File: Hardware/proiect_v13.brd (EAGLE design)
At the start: 160 x 93.7 mm, 103 parts, among them IC1 XC6220A331MR-G, IC2 BD5229G-TR, J1 SAMACSYS_PARTS_USB4110-GF-A, J2 112A-TAAR-R03_ATTEND, J3 FH34SRJ-24S-0.5SH_99_, J4 QWIIC_RIGHT_ANGLE, Q1 20V/4.2A/52mΩ/1.4W, Q2 SI1308EDL-T1-GE3, Q3 20V/4.2A/52mΩ/1.4W, U1 ESP32_WROVER_SPARKFUN-IC-POWE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, U2 ESP32-C6-WROOM-1-N8, U3 ESP32_WROVER_BME680_BME680, U4 MAX17048G+T10, U5 DS3231SN#, U6 W25Q512JVEIQ

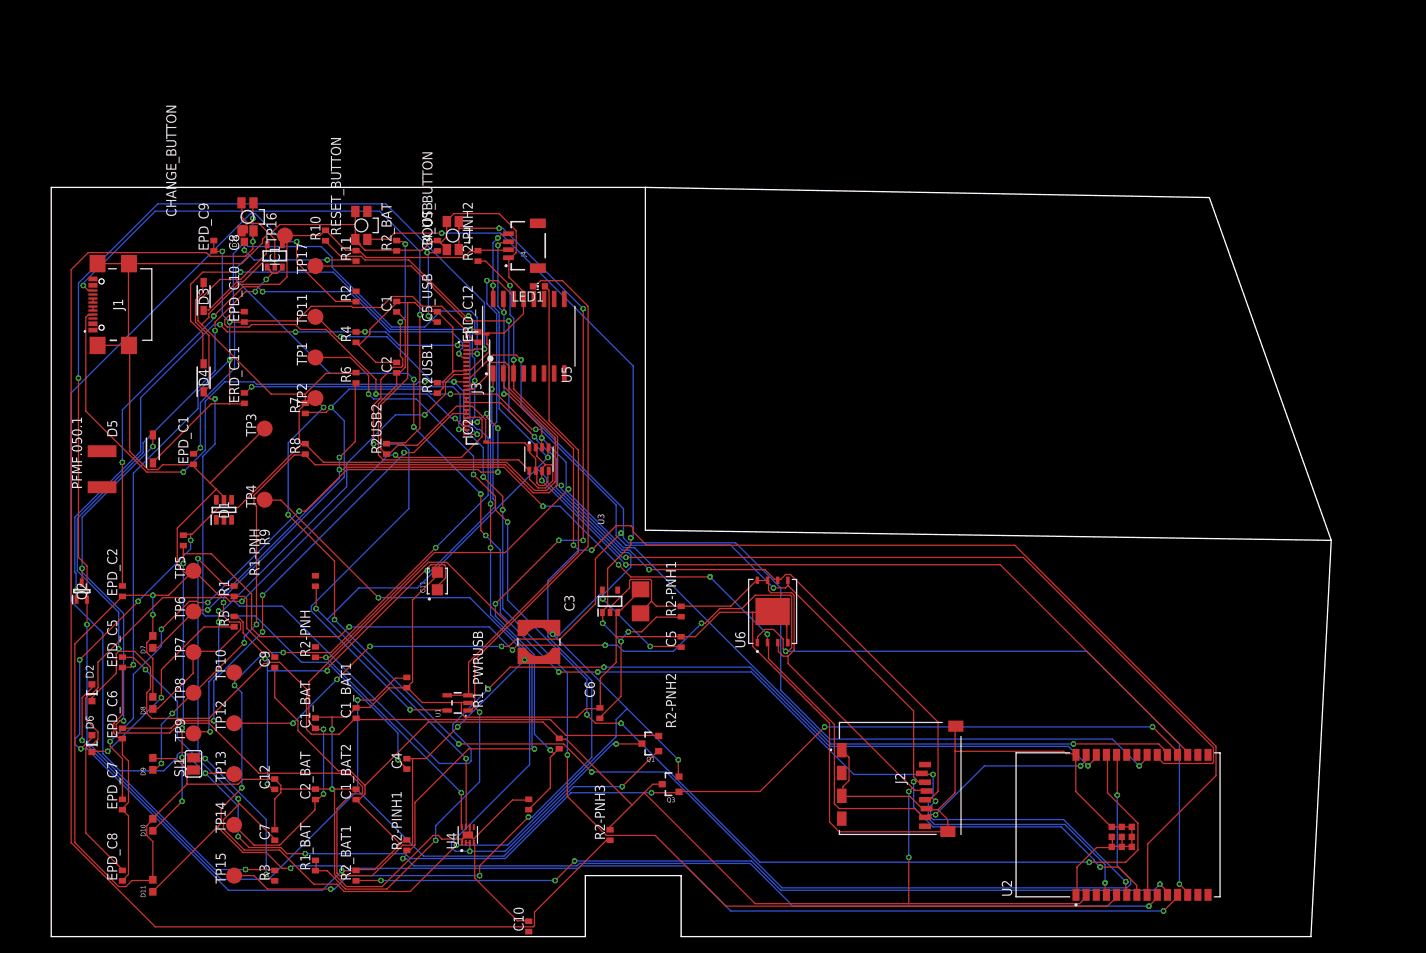
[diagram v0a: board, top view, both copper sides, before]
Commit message: Add files via upload
improved pcb
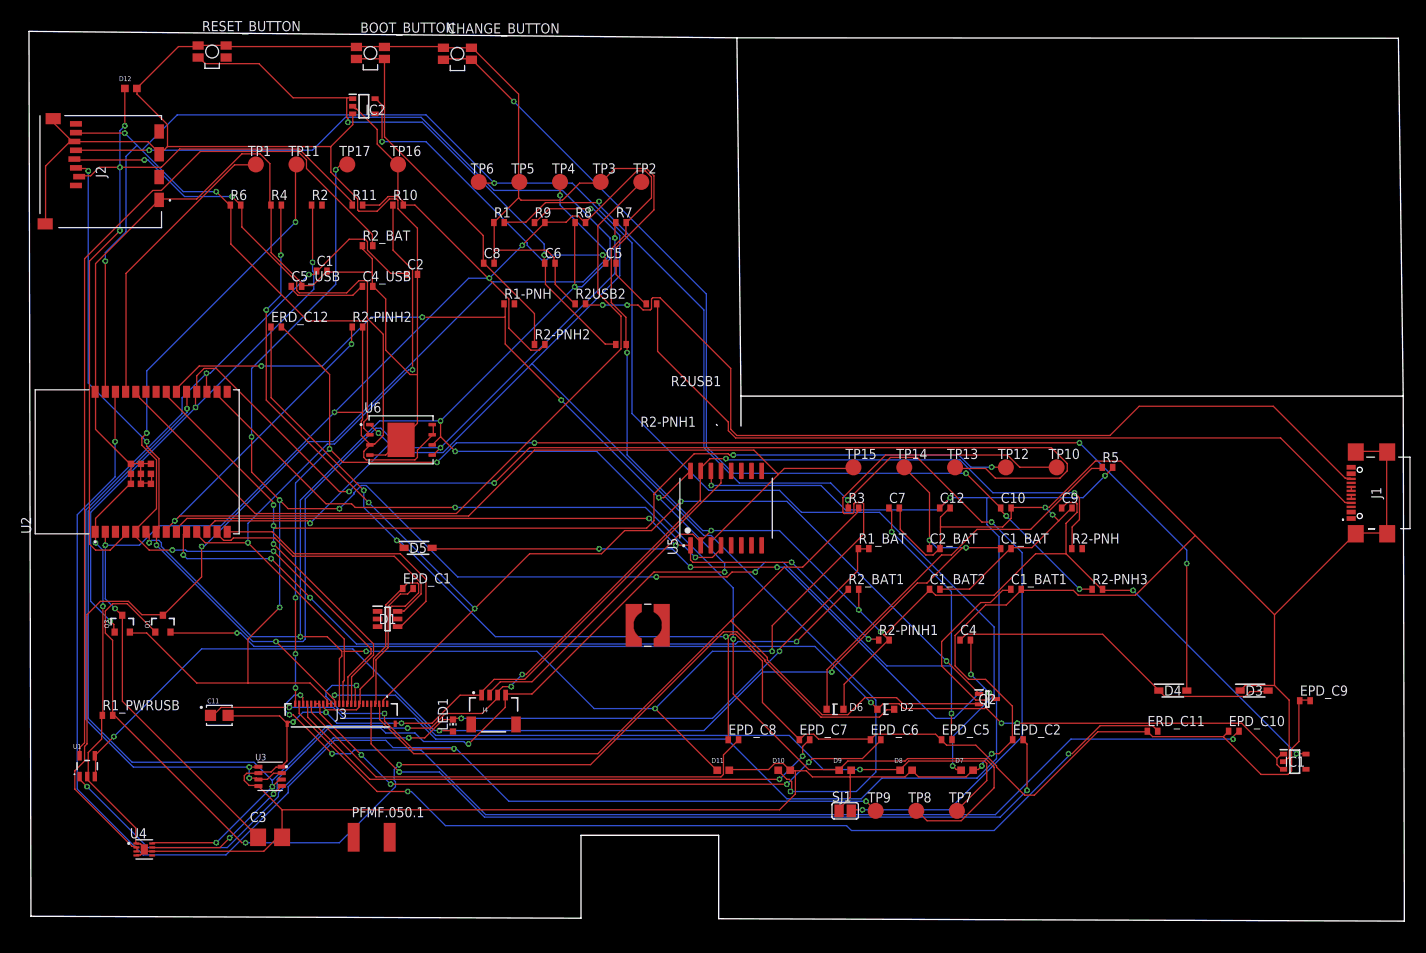
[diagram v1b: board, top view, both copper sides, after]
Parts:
- moved J1 159.0 mm to (168.7, 51.7)
- moved EPD_C9 147.8 mm to (159.2, 25.7), turned to 0 degrees
- moved IC1 142.3 mm to (158.0, 18.1), turned to 0 degrees
- moved D3 140.2 mm to (152.9, 26.9), turned to 0 degrees
- moved J2 139.1 mm to (5.63, 98.9), turned to 270 degrees
- moved EPD_C10 134.1 mm to (150.4, 21.9), turned to 0 degrees
- moved U2 130.7 mm to (13.3, 55.5)
- moved D4 127.3 mm to (142.7, 26.9), turned to 0 degrees
- moved ERD_C11 120.9 mm to (140.2, 21.9), turned to 0 degrees
- moved Q2 114.0 mm to (119.6, 25.9), turned to 0 degrees
- moved EPD_C2 113.5 mm to (123.4, 20.8), turned to 0 degrees
- moved R5 110.9 mm to (134.6, 54.8), turned to 0 degrees
- moved TP10 106.0 mm to (128.2, 54.8), turned to 0 degrees
- moved EPD_C5 103.5 mm to (114.5, 20.8), turned to 0 degrees
- moved D7 103.0 mm to (117.0, 17.0), turned to 0 degrees
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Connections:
- removed net RTC_RTS: U2.16
- removed net USR_D+: U2.14
- removed net USR_D-: U2.13
- net RTC_RST: now also U2.16
- net USB_D+: now also U2.14
- net USB_D-: now also U2.13
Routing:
- net GND: track 689.3 -> 874.1 mm, vias 4 -> 9
- net TX: track 155.1 -> 36.7 mm, vias 6 -> 0
- net PREVGL: track 65.1 -> 183.4 mm, vias 3 -> 8
- net INT_RTC: track 239.4 -> 137.9 mm, vias 7 -> 2
- net MISO: track 167.9 -> 266.3 mm, vias 9 -> 5
- net RESE': track 51.9 -> 148.1 mm, vias 3 -> 4
- net VRTC: track 101.2 -> 196.2 mm, vias 5 -> 4
- net SCK: track 211.5 -> 305.4 mm, vias 8 -> 7
- net N$27: track 40.3 -> 133.9 mm, vias 2 -> 4
- net N$28: track 33.3 -> 120.5 mm
- net GDR: track 75.5 -> 157.3 mm, vias 5 -> 6
- net 32KHZ: track 172.7 -> 96.1 mm, vias 6 -> 4
- net SS_SD: track 178.6 -> 103.6 mm, vias 10 -> 3
- net RTC_RST: track 0.00 -> 72.7 mm, vias 0 -> 2
- net RX: track 162.9 -> 100.0 mm, vias 6 -> 0
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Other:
- board size 160 x 93.7 mm -> 171.9 x 111.2 mm
